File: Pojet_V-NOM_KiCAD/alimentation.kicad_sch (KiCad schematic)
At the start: 2 parts, among them J6 Switch ON/OFF

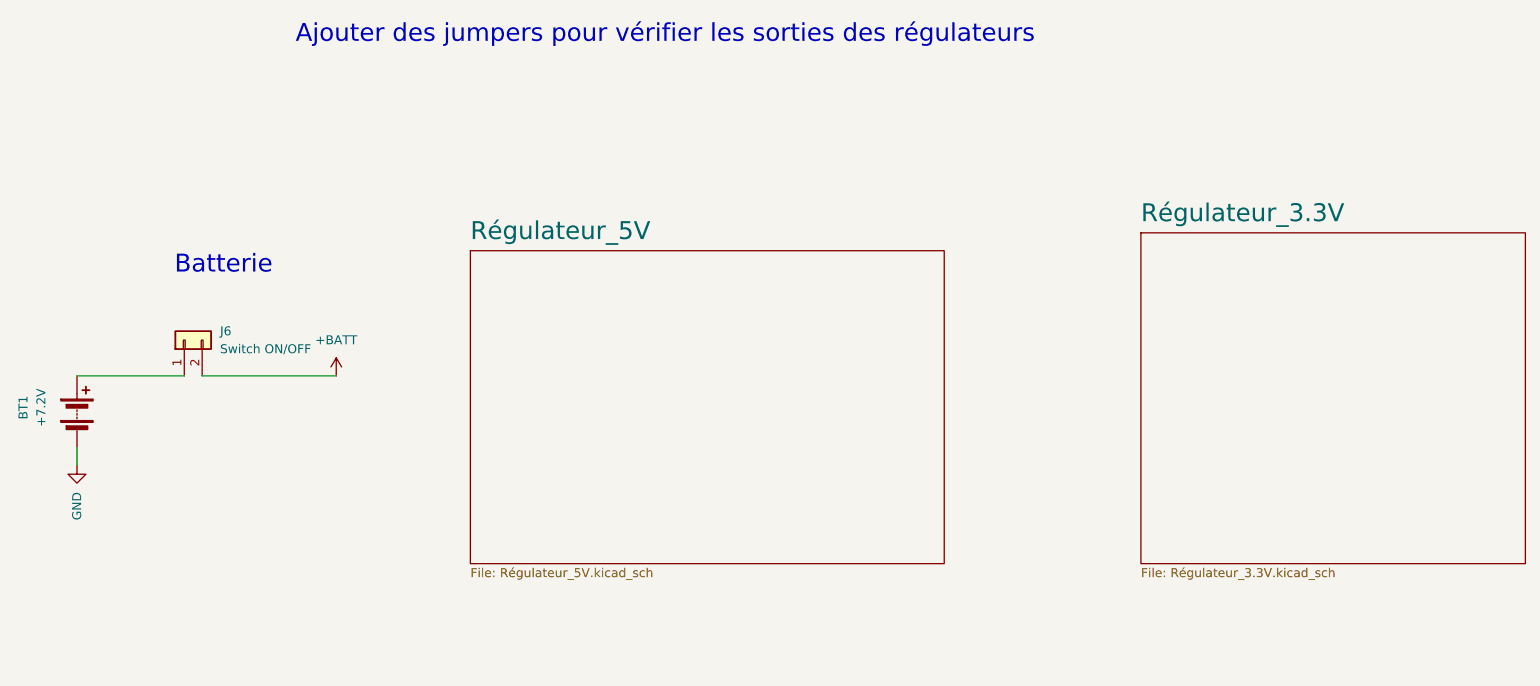
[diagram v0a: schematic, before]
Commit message: Correction des erreurs évidentes
Changements avant vérification des erreurs :
- Désallocation du pin BTN_RESET
- Réarrangement de certaines sources pour cohérence avec tous les
schémas éléctriques
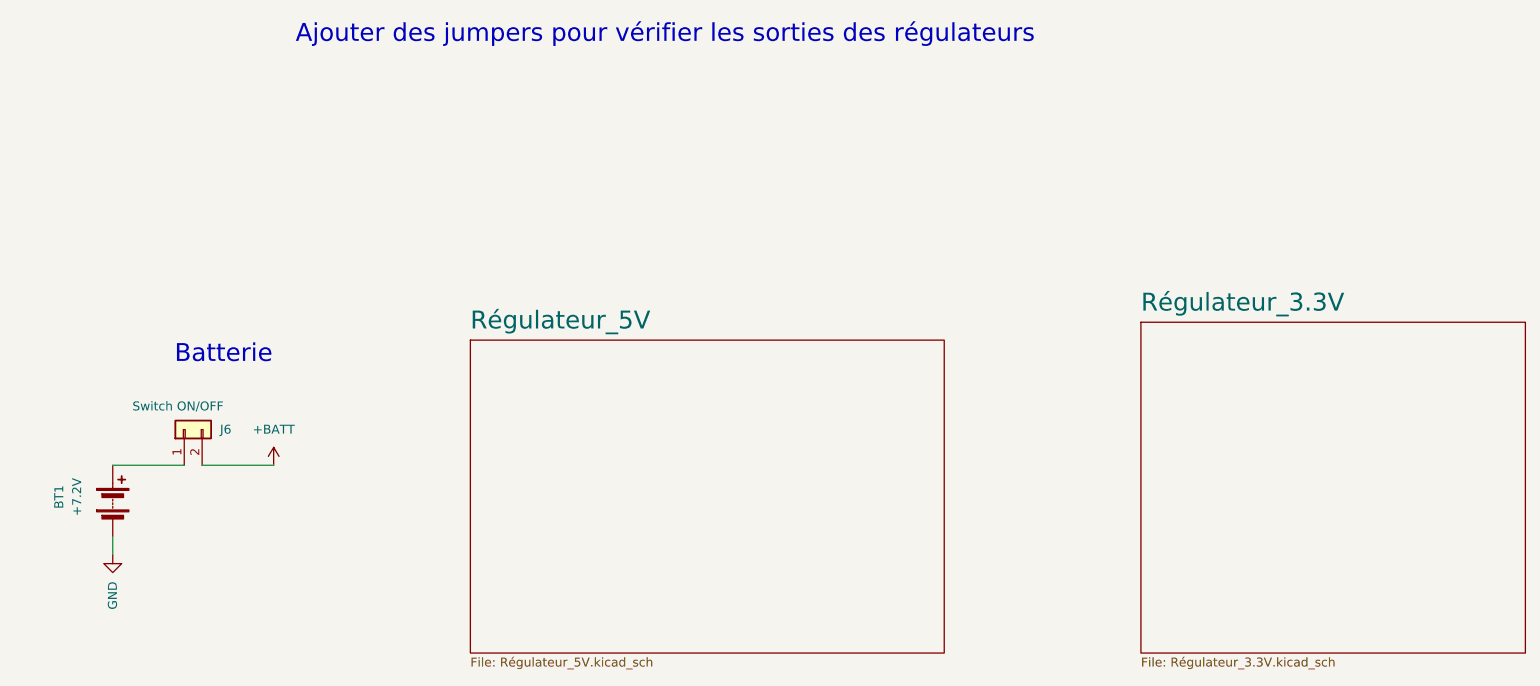
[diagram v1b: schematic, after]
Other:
- moved on the sheet: BT1, J6
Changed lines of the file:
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@@
 	(wire
 		(pts
-			(xy 53.34 83.82) (xy 72.39 83.82)
+			(xy 53.34 96.52) (xy 63.5 96.52)
 		)
 		(stroke
@@
 	(wire
 		(pts
-			(xy 35.56 93.98) (xy 35.56 96.52)
+			(xy 40.64 106.68) (xy 40.64 109.22)
 		)
 		(stroke
@@
 	(wire
 		(pts
-			(xy 35.56 83.82) (xy 50.8 83.82)
+			(xy 40.64 96.52) (xy 50.8 96.52)
 		)
 		(stroke
@@
 	(text "Batterie\n"
 		(exclude_from_sim no)
-		(at 56.388 68.072 0)
+		(at 56.388 80.772 0)
 		(effects
 			(font
@@
 	(symbol
 		(lib_id "power:GND")
-		(at 35.56 96.52 0)
+		(at 40.64 109.22 0)
 		(unit 1)
 		(exclude_from_sim no)
@@
 		(fields_autoplaced yes)
 		(property "Reference" "#PWR0101"
-			(at 35.56 102.87 0)
+			(at 40.64 115.57 0)
 			(effects
 				(font
@@
 		)
 		(property "Value" "GND"
-			(at 35.5599 100.33 90)
+			(at 40.6399 113.03 90)
 			(effects
 				(font
@@
 		)
 		(property "Footprint" ""
-			(at 35.56 96.52 0)
+			(at 40.64 109.22 0)
 			(effects
 				(font
@@
 		)
 		(property "Datasheet" ""
-			(at 35.56 96.52 0)
+			(at 40.64 109.22 0)
 			(effects
 				(font
@@
 		)
 		(property "Description" "Power symbol creates a global label with name \"GND\" , ground"
-			(at 35.56 96.52 0)
+			(at 40.64 109.22 0)
 			(effects
 				(font
@@
 	(symbol
 		(lib_id "Connector_Generic:Conn_01x02")
-		(at 50.8 78.74 90)
+		(at 50.8 91.44 90)
 		(unit 1)
 		(exclude_from_sim no)
@@
 		(on_board yes)
 		(dnp no)
-		(fields_autoplaced yes)
 		(property "Reference" "J6"
-			(at 55.88 77.4699 90)
+			(at 55.88 91.44 90)
 			(effects
 				(font
@@
 		)
 		(property "Value" "Switch ON/OFF"
-			(at 55.88 80.0099 90)
+			(at 43.434 88.138 90)
 			(effects
 				(font
@@
 		)
 		(property "Footprint" "Connector_JST:JST_XH_S2B-XH-A_1x02_P2.50mm_Horizontal"
-			(at 50.8 78.74 0)
+			(at 50.8 91.44 0)
 			(effects
 				(font
@@
 		)
 		(property "Datasheet" "~"
-			(at 50.8 78.74 0)
+			(at 50.8 91.44 0)
 			(effects
 				(font
@@
 		)
 		(property "Description" "Generic connector, single row, 01x02, script generated (kicad-library-utils/schlib/autogen/connector/)"
-			(at 50.8 78.74 0)
+			(at 50.8 91.44 0)
 			(effects
 				(font
@@
 	(symbol
 		(lib_id "power:+BATT")
-		(at 72.39 83.82 0)
+		(at 63.5 96.52 0)
 		(unit 1)
 		(exclude_from_sim no)
@@
 		(fields_autoplaced yes)
 		(property "Reference" "#PWR0401"
-			(at 72.39 87.63 0)
+			(at 63.5 100.33 0)
 			(effects
 				(font
@@
 		)
 		(property "Value" "+BATT"
-			(at 72.39 78.74 0)
+			(at 63.5 91.44 0)
 			(effects
 				(font
@@
 		)
 		(property "Footprint" ""
-			(at 72.39 83.82 0)
+			(at 63.5 96.52 0)
 			(effects
 				(font
@@
 		)
 		(property "Datasheet" ""
-			(at 72.39 83.82 0)
+			(at 63.5 96.52 0)
 			(effects
 				(font
@@
 		)
 		(property "Description" "Power symbol creates a global label with name \"+BATT\""
-			(at 72.39 83.82 0)
+			(at 63.5 96.52 0)
 			(effects
 				(font
@@
 	(symbol
 		(lib_id "Device:Battery")
-		(at 35.56 88.9 0)
+		(at 40.64 101.6 0)
 		(unit 1)
 		(exclude_from_sim no)
@@
 		(fields_autoplaced yes)
 		(property "Reference" "BT1"
-			(at 27.94 88.3285 90)
+			(at 33.02 101.0285 90)
 			(effects
 				(font
@@
 		)
 		(property "Value" "+7.2V"
-			(at 30.48 88.3285 90)
+			(at 35.56 101.0285 90)
 			(effects
 				(font
@@
 		)
 		(property "Footprint" "Connector_JST:JST_XH_S2B-XH-A-1_1x02_P2.50mm_Horizontal"
-			(at 35.56 87.376 90)
+			(at 40.64 100.076 90)
 			(effects
 				(font
@@
 		)
 		(property "Datasheet" "~"
-			(at 35.56 87.376 90)
+			(at 40.64 100.076 90)
 			(effects
 				(font
@@
 		)
 		(property "Description" "Multiple-cell battery"
-			(at 35.56 88.9 0)
+			(at 40.64 101.6 0)
 			(effects
 				(font
@@
 	)
 	(sheet
-		(at 91.44 66.04)
+		(at 91.44 78.74)
 		(size 67.31 44.45)
 		(fields_autoplaced yes)
@@
 		)
 		(property "Sheetname" "Régulateur_5V"
-			(at 91.44 64.6934 0)
+			(at 91.44 77.3934 0)
 			(effects
 				(font
@@
 		)
 		(property "Sheetfile" "Régulateur_5V.kicad_sch"
-			(at 91.44 111.0746 0)
+			(at 91.44 123.7746 0)
 			(effects
 				(font
@@
 	)
 	(sheet
-		(at 186.69 63.5)
+		(at 186.69 76.2)
 		(size 54.61 46.99)
 		(fields_autoplaced yes)
@@
 		)
 		(property "Sheetname" "Régulateur_3.3V"
-			(at 186.69 62.1534 0)
+			(at 186.69 74.8534 0)
 			(effects
 				(font
@@
 		)
 		(property "Sheetfile" "Régulateur_3.3V.kicad_sch"
-			(at 186.69 111.0746 0)
-			(effects
-				(font
+			(at 186.69 123.7746 0)
+			(effects
+				(font
